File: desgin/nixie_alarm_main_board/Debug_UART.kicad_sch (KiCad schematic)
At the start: 1 part, among them J4 JST XH 2.54 3 pin

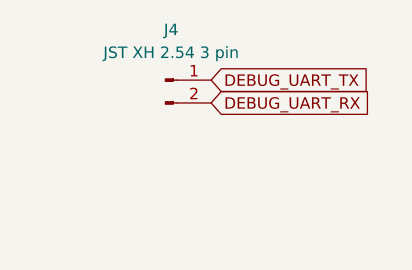
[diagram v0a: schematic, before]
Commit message: copper border
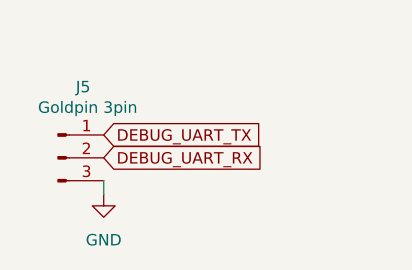
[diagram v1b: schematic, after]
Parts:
- removed J4: JST XH 2.54 3 pin, Connector_JST:JST_EH_S2B-EH_1x02_P2.50mm_Horizontal, symbol Connector:Conn_01x02_Pin
- added J5: Goldpin 3pin, Connector_PinHeader_2.54mm:PinHeader_1x03_P2.54mm_Horizontal, symbol Connector:Conn_01x03_Pin
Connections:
- net DEBUG_UART_RX: now also J5.2 (Pin_2)
- net DEBUG_UART_TX: now also J5.1 (Pin_1)
- new net GND: J5.3 (Pin_3)
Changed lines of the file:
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@@
 	(generator_version "8.0")
 	(paper "A4")
+	(wire
+		(pts
+			(xy 118.618 101.854) (xy 118.618 103.378)
+		)
+		(stroke
+			(width 0)
+			(type default)
+		)
+	)
 	(global_label "DEBUG_UART_RX"
 		(shape input)
-		(at 130.556 93.218 0)
+		(at 118.618 99.314 0)
 		(fields_autoplaced yes)
 		(effects
@@
 		)
 		(property "Intersheetrefs" "${INTERSHEET_REFS}"
-			(at 148.9021 93.218 0)
+			(at 136.9641 99.314 0)
 			(effects
 				(font
@@
 	(global_label "DEBUG_UART_TX"
 		(shape input)
-		(at 130.556 90.678 0)
+		(at 118.618 96.774 0)
 		(fields_autoplaced yes)
 		(effects
@@
 		)
 		(property "Intersheetrefs" "${INTERSHEET_REFS}"
-			(at 148.5997 90.678 0)
+			(at 136.6617 96.774 0)
 			(effects
 				(font
@@
 	)
 	(symbol
-		(lib_id "Connector:Conn_01x02_Pin")
-		(at 125.476 90.678 0)
+		(lib_id "power:GND")
+		(at 118.618 103.378 0)
 		(unit 1)
 		(exclude_from_sim no)
@@
 		(dnp no)
 		(fields_autoplaced yes)
-		(property "Reference" "J4"
-			(at 126.111 85.09 0)
+		(property "Reference" "#PWR041"
+			(at 118.618 109.728 0)
+			(effects
+				(font
+					(size 1.27 1.27)
+				)
+				(hide yes)
+			)
+		)
+		(property "Value" "GND"
+			(at 118.618 108.458 0)
 			(effects
 				(font
@@
 			)
 		)
-		(property "Value" "JST XH 2.54 3 pin"
-			(at 126.111 87.63 0)
+		(property "Footprint" ""
+			(at 118.618 103.378 0)
+			(effects
+				(font
+					(size 1.27 1.27)
+				)
+				(hide yes)
+			)
+		)
+		(property "Datasheet" ""
+			(at 118.618 103.378 0)
+			(effects
+				(font
+					(size 1.27 1.27)
+				)
+				(hide yes)
+			)
+		)
+		(property "Description" "Power symbol creates a global label with name \"GND\" , ground"
+			(at 118.618 103.378 0)
+			(effects
+				(font
+					(size 1.27 1.27)
+				)
+				(hide yes)
+			)
+		)
+		(pin "1"
+		)
+		(instances
+			(project "nixie_alarm_main_board"
+				(path "/a0d555d7-39a0-4a98-b831-70d97d0aa5a1/1fdd9e0c-5909-450c-9e00-c17b847bc6ac"
+					(reference "#PWR041")
+					(unit 1)
+				)
+			)
+		)
+	)
+	(symbol
+		(lib_id "Connector:Conn_01x03_Pin")
+		(at 113.538 99.314 0)
+		(unit 1)
+		(exclude_from_sim no)
+		(in_bom yes)
+		(on_board yes)
+		(dnp no)
+		(property "Reference" "J5"
+			(at 116.332 91.44 0)
 			(effects
 				(font
@@
 			)
 		)
-		(property "Footprint" "Connector_JST:JST_EH_S2B-EH_1x02_P2.50mm_Horizontal"
-			(at 125.476 90.678 0)
+		(property "Value" "Goldpin 3pin "
+			(at 116.84 93.726 0)
+			(effects
+				(font
+					(size 1.27 1.27)
+				)
+			)
+		)
+		(property "Footprint" "Connector_PinHeader_2.54mm:PinHeader_1x03_P2.54mm_Horizontal"
+			(at 113.538 99.314 0)
 			(effects
 				(font
@@
 		)
 		(property "Datasheet" "~"
-			(at 125.476 90.678 0)
+			(at 113.538 99.314 0)
 			(effects
 				(font
@@
 			)
 		)
-		(property "Description" "Generic connector, single row, 01x02, script generated"
-			(at 125.476 90.678 0)
+		(property "Description" "Generic connector, single row, 01x03, script generated"
+			(at 113.538 99.314 0)
 			(effects
 				(font
@@
 		(pin "2"
 		)
+		(pin "3"
+		)
 		(pin "1"
 		)
@@
 			(project "nixie_alarm_main_board"
 				(path "/a0d555d7-39a0-4a98-b831-70d97d0aa5a1/1fdd9e0c-5909-450c-9e00-c17b847bc6ac"
-					(reference "J4")
+					(reference "J5")
 					(unit 1)
 				)
